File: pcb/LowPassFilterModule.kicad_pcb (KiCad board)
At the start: 2 copper layers, 45 x 18 mm, 49 parts, among them J1 SMA, J2 CONN_01X04, J3 SMA, J4 CONN_01X04

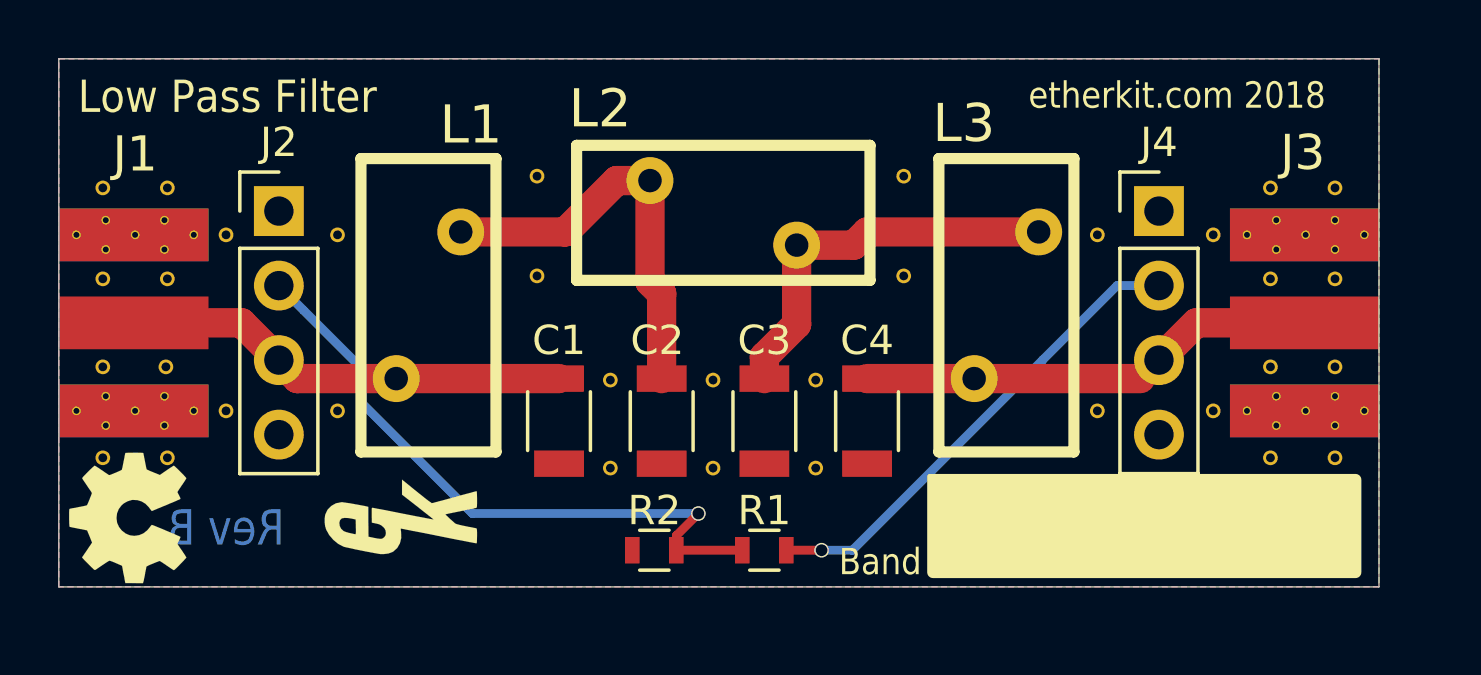
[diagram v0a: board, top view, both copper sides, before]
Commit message: Update for OpenBeacon 2
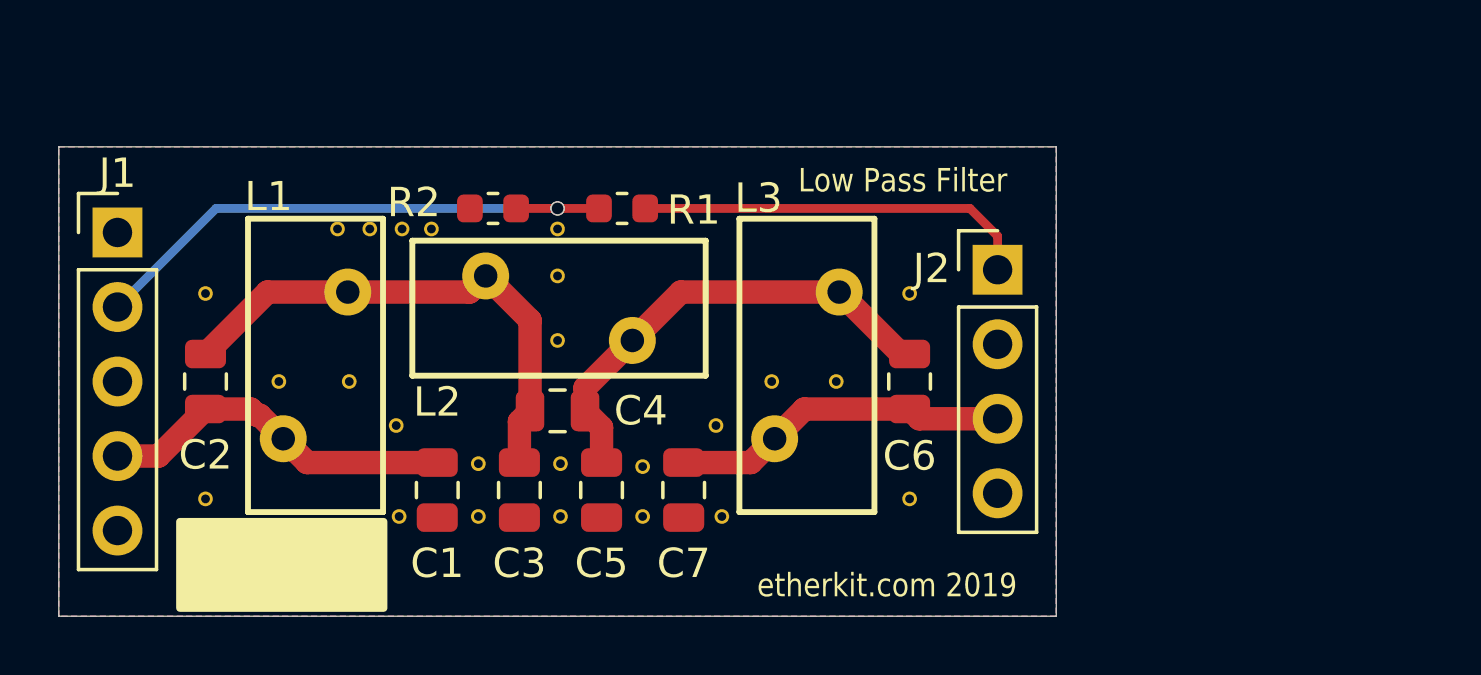
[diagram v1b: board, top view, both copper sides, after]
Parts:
- removed J3: SMA, EtherkitKicadLibrary:SMA-ENDLAUNCH
- removed J4: CONN_01X04, Socket_Strips:Socket_Strip_Straight_1x04_Pitch2.54mm
- removed the VIA at (125.8, 96.0)
- removed the VIA at (143.5, 92.5)
- removed the VIA at (141.3, 92.5)
- removed the VIA at (143.5, 89.5)
- removed the VIA at (141.3, 89.5)
- removed the VIA at (141.3, 86.4)
- removed the VIA at (143.5, 86.4)
- removed the VIA at (143.5, 95.6)
- removed the VIA at (141.3, 95.6)
- removed the VIA at (103.7, 92.5)
- removed the VIA at (101.5, 92.5)
- removed the VIA at (101.5, 89.5)
- removed the VIA at (103.7, 89.5)
- removed the VIA at (103.7, 86.4)
- removed the VIA at (101.5, 86.4)
- added C5: C, Capacitor_SMD:C_0805_2012Metric, F.Cu at (118.5, 96.7)
- added C6: C, Capacitor_SMD:C_0805_2012Metric, F.Cu at (129.0, 93.0)
- added C7: C, Capacitor_SMD:C_0805_2012Metric, F.Cu at (121.3, 96.7)
- added VIA: VAL**, EtherkitKicadLibrary:VIA-05, F.Cu at (117.0, 87.8)
- added VIA: VAL**, EtherkitKicadLibrary:VIA-05, F.Cu at (122.4, 94.5)
- added VIA: VAL**, EtherkitKicadLibrary:VIA-05, F.Cu at (109.5, 87.8)
- added VIA: VAL**, EtherkitKicadLibrary:VIA-05, F.Cu at (110.6, 87.8)
- added VIA: VAL**, EtherkitKicadLibrary:VIA-05, F.Cu at (111.7, 87.8)
- added VIA: VAL**, EtherkitKicadLibrary:VIA-05, F.Cu at (112.7, 87.8)
- C1, C2, C3, C4: footprint Resistors_SMD:R_1206 -> Capacitor_SMD:C_0805_2012Metric
- G***, Ref**: moved to B.Cu
- J1: value SMA -> Conn_01x05; footprint EtherkitKicadLibrary:SMA-ENDLAUNCH -> Connector_PinHeader_2.54mm:PinHeader_1x05_P2.54mm_Vertical
- J2: value CONN_01X04 -> Conn_01x04; footprint Socket_Strips:Socket_Strip_Straight_1x04_Pitch2.54mm -> Connector_PinHeader_2.54mm:PinHeader_1x04_P2.54mm_Vertical
- R1, R2: footprint Resistors_SMD:R_0603 -> Resistor_SMD:R_0603_1608Metric
- moved VIA 34.4 mm to (105.0, 90.0)
- moved VIA 27.5 mm to (129.0, 97.0)
- moved J2 24.6 mm to (132.0, 89.2)
- moved VIA 19.8 mm to (119.9, 97.6)
- moved VIA 18.4 mm to (117.1, 95.8)
- moved VIA 16.2 mm to (122.6, 97.6)
- moved C2 15.6 mm to (105.0, 93.0)
- moved R2 12.9 mm to (114.8, 87.1)
- moved G*** 12.9 mm to (114.2, 92.5), turned to 180 degrees
- moved R1 12.6 mm to (119.2, 87.1)
- moved C4 10.6 mm to (117.0, 94.0), turned to 180 degrees
- moved Ref** 9.62 mm to (107.0, 89.2), turned to 180 degrees
- moved C3 8.67 mm to (115.7, 96.7)
- moved VIA 8.57 mm to (111.6, 97.6)
- moved VIA 8.49 mm to (114.3, 95.8)
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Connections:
- C2 pad 2: GND -> Net-(C1-Pad1)
- C3 pad 1: Net-(C3-Pad1) -> Net-(C2-Pad1)
- C4 pad 2: GND -> Net-(C2-Pad1)
- J1 pad 1: Net-(C1-Pad1) -> GND
- J1 pad 2: GND -> Net-(J1-Pad2)
- J2 pad 1: GND -> VCC
- J2 pad 2: Net-(J2-Pad2) -> GND
- J2 pad 3: Net-(C1-Pad1) -> Net-(C6-Pad1)
- L2 pad 2: Net-(C3-Pad1) -> Net-(C4-Pad1)
- L3 pad 1: Net-(C3-Pad1) -> Net-(C4-Pad1)
- L3 pad 2: Net-(C4-Pad1) -> Net-(C6-Pad1)
- R1 pad 2: Net-(J2-Pad2) -> Net-(J1-Pad2)
- R2 pad 1: Net-(J2-Pad2) -> Net-(J1-Pad2)
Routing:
- net Net-(J2-Pad2): track 22.0 -> 0.00 mm, vias 1 -> 0
- net Net-(J1-Pad2): track 0.00 -> 19.2 mm, vias 0 -> 1
- net Net-(C3-Pad1): track 13.4 -> 0.00 mm
- net Net-(C6-Pad1): track 0.00 -> 11.6 mm
- net Net-(C2-Pad1): track 14.1 -> 17.8 mm
- net Net-(C1-Pad1): track 15.3 -> 12.3 mm
- net VCC: track 16.4 -> 13.6 mm, vias 1 -> 0
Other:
- board size 45 x 18 mm -> 34 x 16 mm
- net class 50ohm: trace_width 1 -> 0.8
- rule trace_min: 0.25 -> 0.2
- rule via_min_size: 0.5 -> 0.4
- board text added: "Rev C"
- board text added: "etherkit.com 2019"
- board text removed: "Rev B"
- board text removed: "etherkit.com 2018"
